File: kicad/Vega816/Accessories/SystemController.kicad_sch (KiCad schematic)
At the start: 3 parts, among them J102 VIA Port

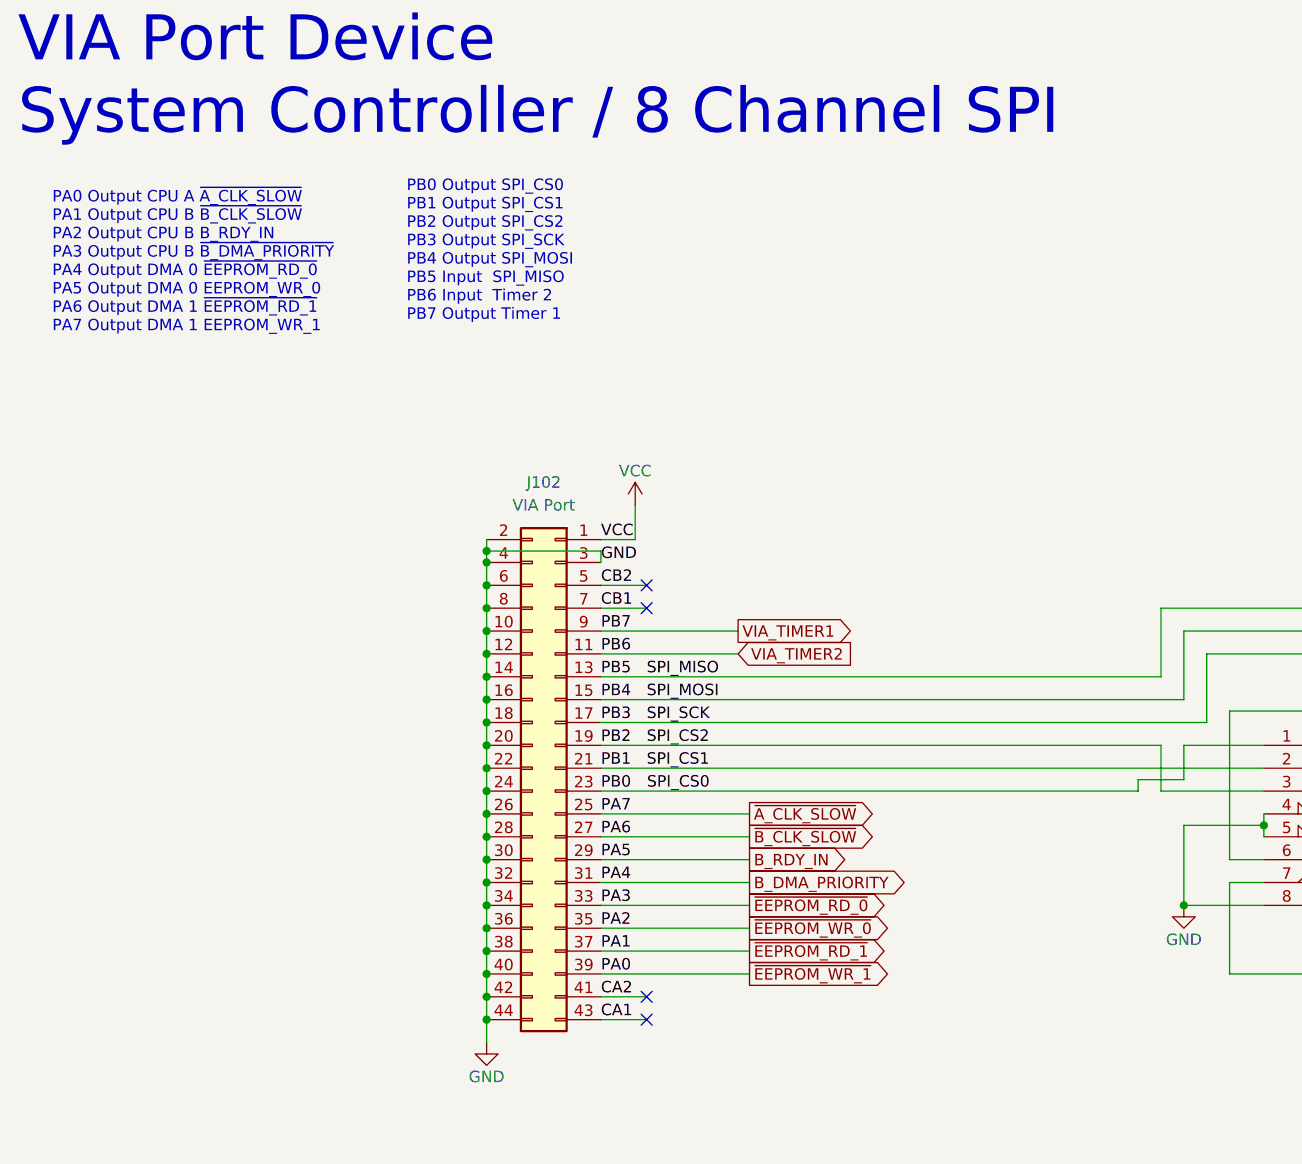
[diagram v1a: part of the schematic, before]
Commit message: expansion port hi ram
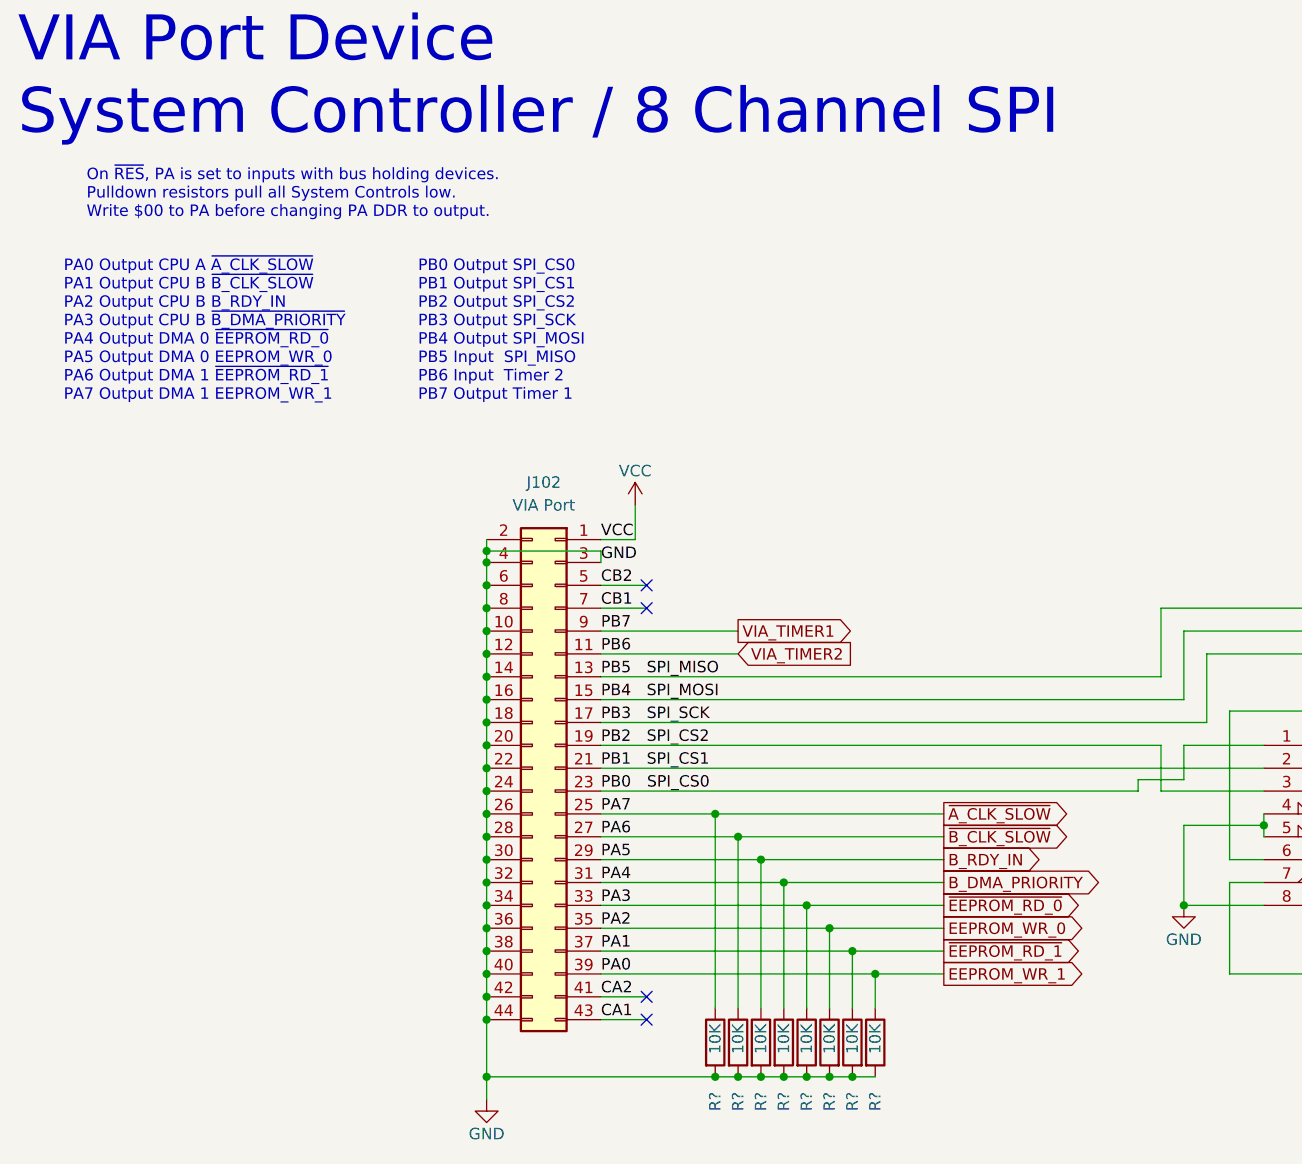
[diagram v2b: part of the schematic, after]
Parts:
- added R? (x8): 10K, symbol Device:R
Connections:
- net B_DMA_PRIORITY: now also R?.1
- net B_RDY_IN: now also R?.1
- net GND: now also R?.2, R?.2, R?.2, R?.2, R?.2, R?.2, R?.2, R?.2
- net ~{A_CLK_SLOW}: now also R?.1
- net ~{B_CLK_SLOW}: now also R?.1
- net ~{EEPROM_RD_0}: now also R?.1
- net ~{EEPROM_RD_1}: now also R?.1
- net ~{EEPROM_WR_0} renamed EEPROM_WR_0
- net EEPROM_WR_0: now also R?.1
- net ~{EEPROM_WR_1} renamed EEPROM_WR_1
- net EEPROM_WR_1: now also R?.1
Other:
- note added: "On ~{RES}, PA is set to inputs with bus holding devices. Pulldown resistors pull all System Controls low. Write $00 to PA before changing PA DDR to output."

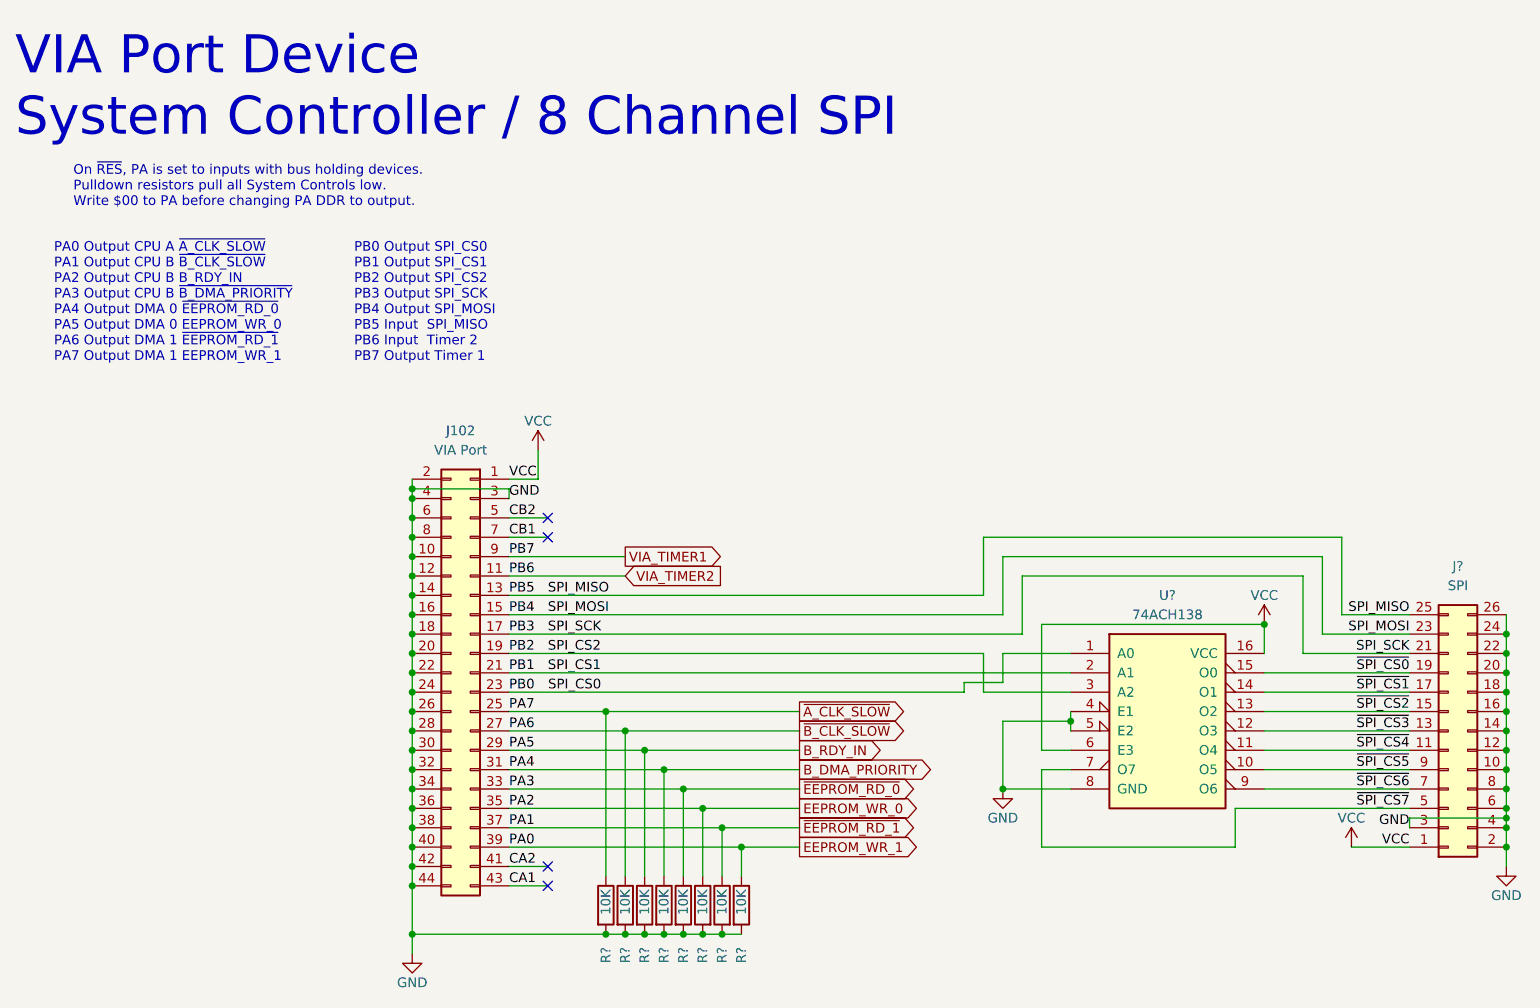
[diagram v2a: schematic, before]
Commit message: new plots
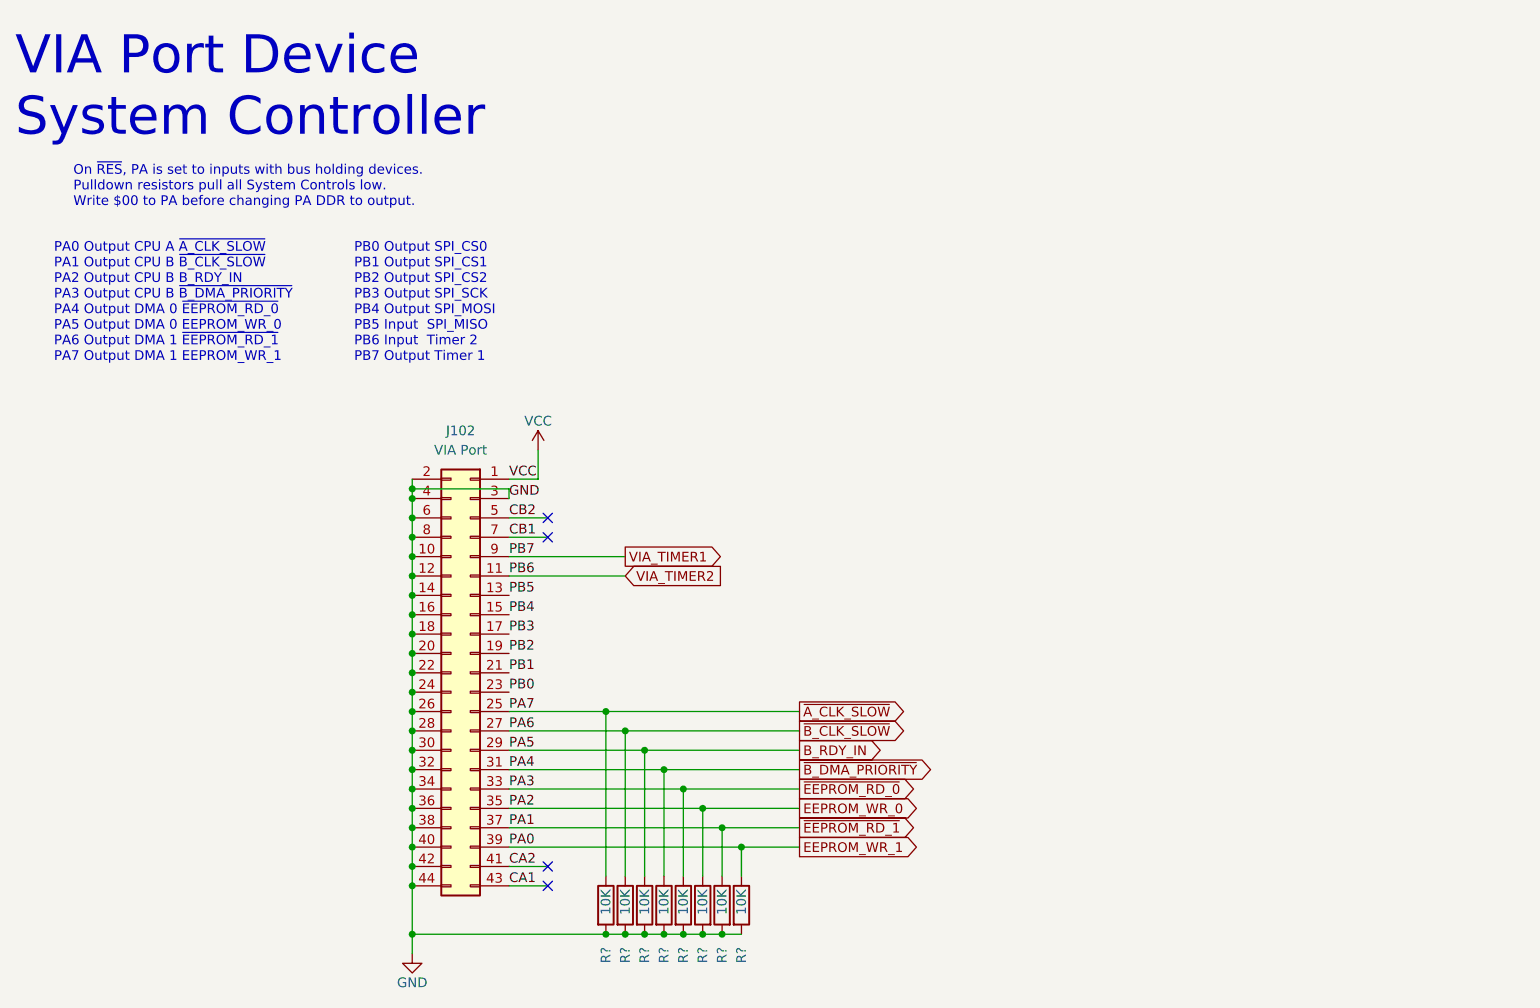
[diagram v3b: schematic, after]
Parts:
- removed J?: SPI, symbol Connector_Generic:Conn_02x13_Odd_Even
- removed U?: 74ACH138, symbol Vega816:74ACH138
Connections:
- net B_DMA_PRIORITY renamed ~{B_DMA_PRIORITY}
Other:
- note added: "VIA Port Device System Controller"
- note removed: "VIA Port Device System Controller / 8 Channel SPI"

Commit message: Big push, Sysctl, DMA Reg
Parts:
- removed R? (x8): 10K, symbol Device:R
- added J1: Sysctrl $7, Connector_PinHeader_2.54mm:PinHeader_2x08_P2.54mm_Vertical, symbol Vega816:Conn_02x08_Odd_Even
- added J10: Sysctrl $A, Connector_PinHeader_2.54mm:PinHeader_2x08_P2.54mm_Vertical, symbol Vega816:Conn_02x08_Odd_Even
- added J11: Sysctrl $B, Connector_PinHeader_2.54mm:PinHeader_2x08_P2.54mm_Vertical, symbol Vega816:Conn_02x08_Odd_Even
- added J12: Sysctrl $C, Connector_PinHeader_2.54mm:PinHeader_2x08_P2.54mm_Vertical, symbol Vega816:Conn_02x08_Odd_Even
- added J13: Sysctrl $D, Connector_PinHeader_2.54mm:PinHeader_2x08_P2.54mm_Vertical, symbol Vega816:Conn_02x08_Odd_Even
- added J16: Sysctrl $E, Connector_PinHeader_2.54mm:PinHeader_2x08_P2.54mm_Vertical, symbol Vega816:Conn_02x08_Odd_Even
- added J17: Sysctrl $F, Connector_PinHeader_2.54mm:PinHeader_2x08_P2.54mm_Vertical, symbol Vega816:Conn_02x08_Odd_Even
- added J18: Sysctrl $8, Connector_PinHeader_2.54mm:PinHeader_2x08_P2.54mm_Vertical, symbol Vega816:Conn_02x08_Odd_Even
- added J2: Sysctrl $6, Connector_PinHeader_2.54mm:PinHeader_2x08_P2.54mm_Vertical, symbol Vega816:Conn_02x08_Odd_Even
- added J3: Sysctrl $5, Connector_PinHeader_2.54mm:PinHeader_2x08_P2.54mm_Vertical, symbol Vega816:Conn_02x08_Odd_Even
- added J4: Sysctrl $4, Connector_PinHeader_2.54mm:PinHeader_2x08_P2.54mm_Vertical, symbol Vega816:Conn_02x08_Odd_Even
- added J5: Sysctrl $3, Connector_PinHeader_2.54mm:PinHeader_2x08_P2.54mm_Vertical, symbol Vega816:Conn_02x08_Odd_Even
- added J6: Sysctrl $2, Connector_PinHeader_2.54mm:PinHeader_2x08_P2.54mm_Vertical, symbol Vega816:Conn_02x08_Odd_Even
- added J7: Sysctrl $1, Connector_PinHeader_2.54mm:PinHeader_2x08_P2.54mm_Vertical, symbol Vega816:Conn_02x08_Odd_Even
- added J8: Sysctrl $0, Connector_PinHeader_2.54mm:PinHeader_2x08_P2.54mm_Vertical, symbol Vega816:Conn_02x08_Odd_Even
- added J9: Sysctrl $9, Connector_PinHeader_2.54mm:PinHeader_2x08_P2.54mm_Vertical, symbol Vega816:Conn_02x08_Odd_Even
- added U11, U18, U22, U32, U49, U53, U57, U6: 74HC32, Package_DIP:DIP-14_W7.62mm_Socket, symbol Vega816:74HC32
- added U15, U20, U30, U47, U5, U51, U55, U59: 74HC259, symbol Vega816:74HC259
- added U17, U48, U60, U63, U67, U70, U73, U?: 74HC373, symbol 74xx:74HC373
- added U2, U3: 74ACH138, Package_DIP:DIP-14_W7.62mm_Socket, symbol Vega816:74ACH138
- added U21, U52, U61, U65, U68, U7, U71, U74: 74HC02, symbol 74xx:74HC02
- added U4: 74HC04, symbol 74xx:74HC04
- added U? (x16): 74HC541, symbol Vega816:74HC541
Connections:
- net GND: now also J10.10 (Pin_10), J10.12 (Pin_12), J10.14 (Pin_14), J10.16 (Pin_16), J10.2 (Pin_2), J10.4 (Pin_4), J10.6 (Pin_6), J10.8 (Pin_8), J11.10 (Pin_10), J11.12 (Pin_12), J11.14 (Pin_14), J11.16 (Pin_16), J11.2 (Pin_2), J11.4 (Pin_4), J11.6 (Pin_6), J11.8 (Pin_8), J12.10 (Pin_10), J12.12 (Pin_12), J12.14 (Pin_14), J12.16 (Pin_16), J12.2 (Pin_2), J12.4 (Pin_4), J12.6 (Pin_6), J12.8 (Pin_8), J13.10 (Pin_10), J13.12 (Pin_12), J13.14 (Pin_14), J13.16 (Pin_16), J13.2 (Pin_2), J13.4 (Pin_4), J13.6 (Pin_6), J13.8 (Pin_8), J16.10 (Pin_10), J16.12 (Pin_12), J16.14 (Pin_14), J16.16 (Pin_16), J16.2 (Pin_2), J16.4 (Pin_4), J16.6 (Pin_6), J16.8 (Pin_8), J17.10 (Pin_10), J17.12 (Pin_12), J17.14 (Pin_14), J17.16 (Pin_16), J17.2 (Pin_2), J17.4 (Pin_4), J17.6 (Pin_6), J17.8 (Pin_8), J18.10 (Pin_10), J18.12 (Pin_12), J18.14 (Pin_14), J18.16 (Pin_16), J18.2 (Pin_2), J18.4 (Pin_4), J18.6 (Pin_6), J18.8 (Pin_8), J4.10 (Pin_10), J4.12 (Pin_12), J4.14 (Pin_14), J4.16 (Pin_16), J4.2 (Pin_2), J4.4 (Pin_4), J4.6 (Pin_6), J4.8 (Pin_8), J8.10 (Pin_10), J8.12 (Pin_12), J8.14 (Pin_14), J8.16 (Pin_16), J8.2 (Pin_2), J8.4 (Pin_4), J8.6 (Pin_6), J8.8 (Pin_8), J9.10 (Pin_10), J9.12 (Pin_12), J9.14 (Pin_14), J9.16 (Pin_16), J9.2 (Pin_2), J9.4 (Pin_4), J9.6 (Pin_6), J9.8 (Pin_8), U15.8 (GND), U17.1 (OE), U17.10 (GND), U20.8 (GND), U30.8 (GND), U47.8 (GND), U48.1 (OE), U48.10 (GND), U5.8 (GND), U51.8 (GND), U55.8 (GND), U59.8 (GND), U60.1 (OE), U60.10 (GND), U63.1 (OE), U63.10 (GND), U67.1 (OE), U67.10 (GND), U70.1 (OE), U70.10 (GND), U73.1 (OE), U73.10 (GND), U?.1 (OE), U?.10 (GND), U?.10 (GND), U?.10 (GND), U?.10 (GND), U?.10 (GND), U?.10 (GND), U?.10 (GND), U?.10 (GND), U?.10 (GND), U?.10 (GND), U?.10 (GND), U?.10 (GND), U?.10 (GND), U?.10 (GND), U?.10 (GND), U?.10 (GND), U?.10 (GND)
- net VCC: now also U15.16 (VCC), U17.20 (VCC), U20.16 (VCC), U30.16 (VCC), U47.16 (VCC), U48.20 (VCC), U5.16 (VCC), U51.16 (VCC), U55.16 (VCC), U59.16 (VCC), U60.20 (VCC), U63.20 (VCC), U67.20 (VCC), U70.20 (VCC), U73.20 (VCC), U?.20 (VCC), U?.20 (VCC), U?.20 (VCC), U?.20 (VCC), U?.20 (VCC), U?.20 (VCC), U?.20 (VCC), U?.20 (VCC), U?.20 (VCC), U?.20 (VCC), U?.20 (VCC), U?.20 (VCC), U?.20 (VCC), U?.20 (VCC), U?.20 (VCC), U?.20 (VCC), U?.20 (VCC)
- net B_RDY_IN renamed PA5
- net PA5: now also U17.14 (D5), U48.14 (D5), U60.14 (D5), U63.14 (D5), U67.14 (D5), U70.14 (D5), U73.14 (D5), U?.13 (Y5), U?.13 (Y5), U?.13 (Y5), U?.13 (Y5), U?.13 (Y5), U?.13 (Y5), U?.13 (Y5), U?.13 (Y5), U?.14 (D5), U?.16 (Y2), U?.16 (Y2), U?.16 (Y2), U?.16 (Y2), U?.16 (Y2), U?.16 (Y2), U?.16 (Y2), U?.16 (Y2)
- net CA2 renamed CA2_~{LE}
- net CA2_~{LE}: now also U11.1, U21.3, U52.3, U6.1, U61.3, U65.3, U68.3, U7.3, U71.3, U74.3
- net CB2 renamed CB2_CLR
- net CB2_CLR: now also U15.15 (Clr), U20.15 (Clr), U30.15 (Clr), U47.15 (Clr), U5.15 (Clr), U51.15 (Clr), U55.15 (Clr), U59.15 (Clr)
- net EEPROM_WR_0 renamed PA2
- net PA2: now also U17.7 (D2), U48.7 (D2), U60.7 (D2), U63.7 (D2), U67.7 (D2), U70.7 (D2), U73.7 (D2), U?.13 (Y5), U?.13 (Y5), U?.13 (Y5), U?.13 (Y5), U?.13 (Y5), U?.13 (Y5), U?.13 (Y5), U?.13 (Y5), U?.16 (Y2), U?.16 (Y2), U?.16 (Y2), U?.16 (Y2), U?.16 (Y2), U?.16 (Y2), U?.16 (Y2), U?.16 (Y2), U?.7 (D2)
- net EEPROM_WR_1 renamed PA0_D
- net PA0_D: now also U15.13 (D), U17.3 (D0), U20.13 (D), U30.13 (D), U47.13 (D), U48.3 (D0), U5.13 (D), U51.13 (D), U55.13 (D), U59.13 (D), U60.3 (D0), U63.3 (D0), U67.3 (D0), U70.3 (D0), U73.3 (D0), U?.11 (Y7), U?.11 (Y7), U?.11 (Y7), U?.11 (Y7), U?.11 (Y7), U?.11 (Y7), U?.11 (Y7), U?.11 (Y7), U?.18 (Y0), U?.18 (Y0), U?.18 (Y0), U?.18 (Y0), U?.18 (Y0), U?.18 (Y0), U?.18 (Y0), U?.18 (Y0), U?.3 (D0)
- net PB0 renamed PB0_A0
- net PB0_A0: now also U15.1 (A0), U20.1 (A0), U30.1 (A0), U47.1 (A0), U5.1 (A0), U51.1 (A0), U55.1 (A0), U59.1 (A0)
- net PB1 renamed PB1_A1
- net PB1_A1: now also U15.2 (A1), U20.2 (A1), U30.2 (A1), U47.2 (A1), U5.2 (A1), U51.2 (A1), U55.2 (A1), U59.2 (A1)
- net PB2 renamed PB2_A2
- net PB2_A2: now also U15.3 (A2), U20.3 (A2), U30.3 (A2), U47.3 (A2), U5.3 (A2), U51.3 (A2), U55.3 (A2), U59.3 (A2)
- net PB3 renamed PB3_A3
- net PB3_A3: now also U2.1 (A0), U3.1 (A0)
- net PB4 renamed PB4_A4
- net PB4_A4: now also U2.2 (A1), U3.2 (A1)
- net PB5 renamed PB5_A5
- net PB5_A5: now also U2.3 (A2), U3.3 (A2)
- net VIA_TIMER1 renamed PB7_RD
- net PB7_RD: now also U4.1
- net VIA_TIMER2 renamed PB6_A6
- net PB6_A6: now also U2.4 (E1), U3.6 (E3)
- net ~{A_CLK_SLOW} renamed PA7
- net PA7: now also U17.18 (D7), U48.18 (D7), U60.18 (D7), U63.18 (D7), U67.18 (D7), U70.18 (D7), U73.18 (D7), U?.11 (Y7), U?.11 (Y7), U?.11 (Y7), U?.11 (Y7), U?.11 (Y7), U?.11 (Y7), U?.11 (Y7), U?.11 (Y7), U?.18 (D7), U?.18 (Y0), U?.18 (Y0), U?.18 (Y0), U?.18 (Y0), U?.18 (Y0), U?.18 (Y0), U?.18 (Y0), U?.18 (Y0)
- net ~{B_CLK_SLOW} renamed PA6
- net PA6: now also U17.17 (D6), U48.17 (D6), U60.17 (D6), U63.17 (D6), U67.17 (D6), U70.17 (D6), U73.17 (D6), U?.12 (Y6), U?.12 (Y6), U?.12 (Y6), U?.12 (Y6), U?.12 (Y6), U?.12 (Y6), U?.12 (Y6), U?.12 (Y6), U?.17 (D6), U?.17 (Y1), U?.17 (Y1), U?.17 (Y1), U?.17 (Y1), U?.17 (Y1), U?.17 (Y1), U?.17 (Y1), U?.17 (Y1)
- net ~{B_DMA_PRIORITY} renamed PA4
- net PA4: now also U17.13 (D4), U48.13 (D4), U60.13 (D4), U63.13 (D4), U67.13 (D4), U70.13 (D4), U73.13 (D4), U?.13 (D4), U?.14 (Y4), U?.14 (Y4), U?.14 (Y4), U?.14 (Y4), U?.14 (Y4), U?.14 (Y4), U?.14 (Y4), U?.14 (Y4), U?.15 (Y3), U?.15 (Y3), U?.15 (Y3), U?.15 (Y3), U?.15 (Y3), U?.15 (Y3), U?.15 (Y3), U?.15 (Y3)
- net ~{EEPROM_RD_0} renamed PA3
- net PA3: now also U17.8 (D3), U48.8 (D3), U60.8 (D3), U63.8 (D3), U67.8 (D3), U70.8 (D3), U73.8 (D3), U?.14 (Y4), U?.14 (Y4), U?.14 (Y4), U?.14 (Y4), U?.14 (Y4), U?.14 (Y4), U?.14 (Y4), U?.14 (Y4), U?.15 (Y3), U?.15 (Y3), U?.15 (Y3), U?.15 (Y3), U?.15 (Y3), U?.15 (Y3), U?.15 (Y3), U?.15 (Y3), U?.8 (D3)
- net ~{EEPROM_RD_1} renamed PA1
- net PA1: now also U17.4 (D1), U48.4 (D1), U60.4 (D1), U63.4 (D1), U67.4 (D1), U70.4 (D1), U73.4 (D1), U?.12 (Y6), U?.12 (Y6), U?.12 (Y6), U?.12 (Y6), U?.12 (Y6), U?.12 (Y6), U?.12 (Y6), U?.12 (Y6), U?.17 (Y1), U?.17 (Y1), U?.17 (Y1), U?.17 (Y1), U?.17 (Y1), U?.17 (Y1), U?.17 (Y1), U?.17 (Y1), U?.4 (D1)
- new net: J5.1 (Pin_1), U47.12 (Q7)
- new net: J5.10 (Pin_10), U?.5 (A3)
- new net: J5.11 (Pin_11), U47.6 (Q2)
- new net: J5.12 (Pin_12), U?.4 (A2)
- new net: J5.13 (Pin_13), U47.5 (Q1)
- new net: J5.14 (Pin_14), U?.3 (A1)
- new net: J5.15 (Pin_15), U47.4 (Q0)
- new net: J5.16 (Pin_16), U?.2 (A0)
- new net: J5.2 (Pin_2), U?.9 (A7)
- new net: J5.3 (Pin_3), U47.11 (Q6)
- new net: J5.4 (Pin_4), U?.8 (A6)
- new net: J5.5 (Pin_5), U47.10 (Q5)
- new net: J5.6 (Pin_6), U?.7 (A5)
- new net: J5.7 (Pin_7), U47.9 (Q4)
- new net: J5.8 (Pin_8), U?.6 (A4)
- new net: J5.9 (Pin_9), U47.7 (Q3)
- new net: U2.14 (O1), U53.2, U?.1 (G1)
- new net: U4.2, U?.19 (G2), U?.19 (G2), U?.19 (G2), U?.19 (G2), U?.19 (G2), U?.19 (G2), U?.19 (G2), U?.19 (G2), U?.19 (G2), U?.19 (G2), U?.19 (G2), U?.19 (G2), U?.19 (G2), U?.19 (G2), U?.19 (G2), U?.19 (G2)
- new net: J7.16 (Pin_16), U?.2 (A0)
- new net: J7.14 (Pin_14), U?.3 (A1)
- new net: J7.12 (Pin_12), U?.4 (A2)
- new net: J7.10 (Pin_10), U?.5 (A3)
- new net: J7.8 (Pin_8), U?.6 (A4)
- new net: J7.6 (Pin_6), U?.7 (A5)
- new net: J7.4 (Pin_4), U?.8 (A6)
- new net: J7.2 (Pin_2), U?.9 (A7)
- new net: U3.15 (O0), U7.2, U?.1 (G1)
- new net: J18.1 (Pin_1), U?.2 (A0), U?.2 (O0)
- new net: J18.3 (Pin_3), U?.3 (A1), U?.5 (O1)
- new net: J18.5 (Pin_5), U?.4 (A2), U?.6 (O2)
- new net: J18.7 (Pin_7), U?.5 (A3), U?.9 (O3)
- new net: J18.9 (Pin_9), U?.12 (O4), U?.6 (A4)
- new net: J18.11 (Pin_11), U?.15 (O5), U?.7 (A5)
- new net: J18.13 (Pin_13), U?.16 (O6), U?.8 (A6)
- new net: J18.15 (Pin_15), U?.19 (O7), U?.9 (A7)
- new net: U60.11 (LE), U61.1
- new net: J11.9 (Pin_9), U60.12 (O4), U?.6 (A4)
- new net: J11.11 (Pin_11), U60.15 (O5), U?.7 (A5)
- new net: J11.13 (Pin_13), U60.16 (O6), U?.8 (A6)
- new net: J11.15 (Pin_15), U60.19 (O7), U?.9 (A7)
- new net: J11.1 (Pin_1), U60.2 (O0), U?.2 (A0)
- new net: J11.3 (Pin_3), U60.5 (O1), U?.3 (A1)
- new net: J11.5 (Pin_5), U60.6 (O2), U?.4 (A2)
- new net: J11.7 (Pin_7), U60.9 (O3), U?.5 (A3)
- new net: U11.2, U2.9 (O6), U?.1 (G1)
- new net: U11.3, U15.14 (E)
- new net: U17.11 (LE), U21.1
- new net: J9.9 (Pin_9), U17.12 (O4), U?.6 (A4)
- new net: J9.11 (Pin_11), U17.15 (O5), U?.7 (A5)
- new net: J9.13 (Pin_13), U17.16 (O6), U?.8 (A6)
- new net: J9.15 (Pin_15), U17.19 (O7), U?.9 (A7)
- new net: J9.1 (Pin_1), U17.2 (O0), U?.2 (A0)
- new net: J9.3 (Pin_3), U17.5 (O1), U?.3 (A1)
- new net: J9.5 (Pin_5), U17.6 (O2), U?.4 (A2)
- new net: J9.7 (Pin_7), U17.9 (O3), U?.5 (A3)
- new net: U18.2, U2.10 (O5), U?.1 (G1)
- new net: U2.11 (O4), U22.2, U?.1 (G1)
- new net: U2.12 (O3), U32.2, U?.1 (G1)
- new net: U2.13 (O2), U49.2, U?.1 (G1)
- new net: U2.15 (O0), U57.2, U?.1 (G1)
- new net: U2.16 (VCC), U2.6 (E3)
- new net: U2.5 (E2), U2.8 (GND)
- new net: U2.7 (O7), U6.2, U?.1 (G1)
- new net: J7.1 (Pin_1), U55.12 (Q7)
- new net: J7.11 (Pin_11), U55.6 (Q2)
- new net: J7.13 (Pin_13), U55.5 (Q1)
- new net: J7.15 (Pin_15), U55.4 (Q0)
- new net: J7.3 (Pin_3), U55.11 (Q6)
- new net: J7.5 (Pin_5), U55.10 (Q5)
- new net: J7.7 (Pin_7), U55.9 (Q4)
- new net: J7.9 (Pin_9), U55.7 (Q3)
- new net: U18.1, U22.1, U32.1, U49.1
- new net: U22.3, U30.14 (E)
- new net: U3.10 (O5), U68.2, U?.1 (G1)
- new net: J13.1 (Pin_1), U67.2 (O0), U?.2 (A0)
- new net: J13.3 (Pin_3), U67.5 (O1), U?.3 (A1)
- new net: J13.5 (Pin_5), U67.6 (O2), U?.4 (A2)
- new net: J13.7 (Pin_7), U67.9 (O3), U?.5 (A3)
- new net: J13.9 (Pin_9), U67.12 (O4), U?.6 (A4)
- new net: J13.11 (Pin_11), U67.15 (O5), U?.7 (A5)
- new net: J13.13 (Pin_13), U67.16 (O6), U?.8 (A6)
- new net: J13.15 (Pin_15), U67.19 (O7), U?.9 (A7)
- new net: J2.16 (Pin_16), U?.2 (A0)
- new net: J2.14 (Pin_14), U?.3 (A1)
- new net: J2.12 (Pin_12), U?.4 (A2)
- new net: J2.10 (Pin_10), U?.5 (A3)
- new net: J2.8 (Pin_8), U?.6 (A4)
- new net: J2.6 (Pin_6), U?.7 (A5)
- new net: J2.4 (Pin_4), U?.8 (A6)
- new net: J2.2 (Pin_2), U?.9 (A7)
- new net: U21.2, U3.14 (O1), U?.1 (G1)
- new net: J2.5 (Pin_5), U15.10 (Q5)
- new net: J2.3 (Pin_3), U15.11 (Q6)
- new net: J2.1 (Pin_1), U15.12 (Q7)
- new net: J2.15 (Pin_15), U15.4 (Q0)
- new net: J2.13 (Pin_13), U15.5 (Q1)
- new net: J2.11 (Pin_11), U15.6 (Q2)
- new net: J2.9 (Pin_9), U15.7 (Q3)
- new net: J2.7 (Pin_7), U15.9 (Q4)
- new net: U3.12 (O3), U61.2, U?.1 (G1)
- new net: U53.1, U57.1
- new net: U53.3, U55.14 (E)
- new net: J8.15 (Pin_15), U59.4 (Q0), U?.2 (A0)
- new net: J8.13 (Pin_13), U59.5 (Q1), U?.3 (A1)
- new net: J8.11 (Pin_11), U59.6 (Q2), U?.4 (A2)
- new net: J8.9 (Pin_9), U59.7 (Q3), U?.5 (A3)
- new net: J8.7 (Pin_7), U59.9 (Q4), U?.6 (A4)
- new net: J8.5 (Pin_5), U59.10 (Q5), U?.7 (A5)
- new net: J8.3 (Pin_3), U59.11 (Q6), U?.8 (A6)
- new net: J8.1 (Pin_1), U59.12 (Q7), U?.9 (A7)
- new net: U67.11 (LE), U68.1
- new net: U18.3, U20.14 (E)
- new net: U32.3, U47.14 (E)
- new net: U3.9 (O6), U71.2, U?.1 (G1)
- new net: J16.1 (Pin_1), U70.2 (O0), U?.2 (A0)
- new net: J16.3 (Pin_3), U70.5 (O1), U?.3 (A1)
- new net: J16.5 (Pin_5), U70.6 (O2), U?.4 (A2)
- new net: J16.7 (Pin_7), U70.9 (O3), U?.5 (A3)
- new net: J16.9 (Pin_9), U70.12 (O4), U?.6 (A4)
- new net: J16.11 (Pin_11), U70.15 (O5), U?.7 (A5)
- new net: J16.13 (Pin_13), U70.16 (O6), U?.8 (A6)
- new net: J16.15 (Pin_15), U70.19 (O7), U?.9 (A7)
- new net: J12.1 (Pin_1), U63.2 (O0), U?.2 (A0)
- new net: J12.11 (Pin_11), U63.15 (O5), U?.7 (A5)
- new net: J12.13 (Pin_13), U63.16 (O6), U?.8 (A6)
- new net: J12.15 (Pin_15), U63.19 (O7), U?.9 (A7)
- new net: J12.3 (Pin_3), U63.5 (O1), U?.3 (A1)
- new net: J12.5 (Pin_5), U63.6 (O2), U?.4 (A2)
- new net: J12.7 (Pin_7), U63.9 (O3), U?.5 (A3)
- new net: J12.9 (Pin_9), U63.12 (O4), U?.6 (A4)
- new net: J6.1 (Pin_1), U51.12 (Q7)
- new net: J6.10 (Pin_10), U?.5 (A3)
- new net: J6.11 (Pin_11), U51.6 (Q2)
- new net: J6.12 (Pin_12), U?.4 (A2)
- new net: J6.13 (Pin_13), U51.5 (Q1)
- new net: J6.14 (Pin_14), U?.3 (A1)
- new net: J6.15 (Pin_15), U51.4 (Q0)
- new net: J6.16 (Pin_16), U?.2 (A0)
- new net: J6.2 (Pin_2), U?.9 (A7)
- new net: J6.3 (Pin_3), U51.11 (Q6)
- new net: J6.4 (Pin_4), U?.8 (A6)
- new net: J6.5 (Pin_5), U51.10 (Q5)
- new net: J6.6 (Pin_6), U?.7 (A5)
- new net: J6.7 (Pin_7), U51.9 (Q4)
- new net: J6.8 (Pin_8), U?.6 (A4)
- new net: J6.9 (Pin_9), U51.7 (Q3)
- new net: J10.1 (Pin_1), U48.2 (O0), U?.2 (A0)
- new net: J10.11 (Pin_11), U48.15 (O5), U?.7 (A5)
- new net: J10.13 (Pin_13), U48.16 (O6), U?.8 (A6)
- new net: J10.15 (Pin_15), U48.19 (O7), U?.9 (A7)
- new net: J10.3 (Pin_3), U48.5 (O1), U?.3 (A1)
- new net: J10.5 (Pin_5), U48.6 (O2), U?.4 (A2)
- new net: J10.7 (Pin_7), U48.9 (O3), U?.5 (A3)
- new net: J10.9 (Pin_9), U48.12 (O4), U?.6 (A4)
- new net: J3.1 (Pin_1), U20.12 (Q7)
- new net: J3.10 (Pin_10), U?.5 (A3)
- new net: J3.11 (Pin_11), U20.6 (Q2)
- new net: J3.12 (Pin_12), U?.4 (A2)
- new net: J3.13 (Pin_13), U20.5 (Q1)
- new net: J3.14 (Pin_14), U?.3 (A1)
- new net: J3.15 (Pin_15), U20.4 (Q0)
- new net: J3.16 (Pin_16), U?.2 (A0)
- new net: J3.2 (Pin_2), U?.9 (A7)
- new net: J3.3 (Pin_3), U20.11 (Q6)
- new net: J3.4 (Pin_4), U?.8 (A6)
- new net: J3.5 (Pin_5), U20.10 (Q5)
- new net: J3.6 (Pin_6), U?.7 (A5)
- new net: J3.7 (Pin_7), U20.9 (Q4)
- new net: J3.8 (Pin_8), U?.6 (A4)
- new net: J3.9 (Pin_9), U20.7 (Q3)
- new net: U48.11 (LE), U52.1
- new net: U57.3, U59.14 (E)
- new net: J1.16 (Pin_16), U?.2 (A0)
- new net: J1.14 (Pin_14), U?.3 (A1)
- new net: J1.12 (Pin_12), U?.4 (A2)
- new net: J1.10 (Pin_10), U?.5 (A3)
- new net: J1.8 (Pin_8), U?.6 (A4)
- new net: J1.6 (Pin_6), U?.7 (A5)
- new net: J1.4 (Pin_4), U?.8 (A6)
- new net: J1.2 (Pin_2), U?.9 (A7)
- new net: U7.1, U?.11 (LE)
- new net: J4.1 (Pin_1), U30.12 (Q7), U?.9 (A7)
- new net: J4.11 (Pin_11), U30.6 (Q2), U?.4 (A2)
- new net: J4.13 (Pin_13), U30.5 (Q1), U?.3 (A1)
- new net: J4.15 (Pin_15), U30.4 (Q0), U?.2 (A0)
- new net: J4.3 (Pin_3), U30.11 (Q6), U?.8 (A6)
- new net: J4.5 (Pin_5), U30.10 (Q5), U?.7 (A5)
- new net: J4.7 (Pin_7), U30.9 (Q4), U?.6 (A4)
- new net: J4.9 (Pin_9), U30.7 (Q3), U?.5 (A3)
- new net: U3.11 (O4), U65.2, U?.1 (G1)
- new net: U3.7 (O7), U74.2, U?.1 (G1)
- new net: J17.1 (Pin_1), U73.2 (O0), U?.2 (A0)
- new net: J17.3 (Pin_3), U73.5 (O1), U?.3 (A1)
- new net: J17.5 (Pin_5), U73.6 (O2), U?.4 (A2)
- new net: J17.7 (Pin_7), U73.9 (O3), U?.5 (A3)
- new net: J17.9 (Pin_9), U73.12 (O4), U?.6 (A4)
- new net: J17.11 (Pin_11), U73.15 (O5), U?.7 (A5)
- new net: J17.13 (Pin_13), U73.16 (O6), U?.8 (A6)
- new net: J17.15 (Pin_15), U73.19 (O7), U?.9 (A7)
- new net: U3.13 (O2), U52.2, U?.1 (G1)
- new net: U3.4 (E1), U3.5 (E2), U3.8 (GND)
- new net: U63.11 (LE), U65.1
- new net: J1.1 (Pin_1), U5.12 (Q7)
- new net: J1.11 (Pin_11), U5.6 (Q2)
- new net: J1.13 (Pin_13), U5.5 (Q1)
- new net: J1.15 (Pin_15), U5.4 (Q0)
- new net: J1.3 (Pin_3), U5.11 (Q6)
- new net: J1.5 (Pin_5), U5.10 (Q5)
- new net: J1.7 (Pin_7), U5.9 (Q4)
- new net: J1.9 (Pin_9), U5.7 (Q3)
- new net: U70.11 (LE), U71.1
- new net: U49.3, U51.14 (E)
- new net: U73.11 (LE), U74.1
- new net: U5.14 (E), U6.3
- no-connect marks 4 -> 2
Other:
- note added: "Sysctrl Registers 16 x 8 bit latches (8 addressable) VIA Port Device"
- note removed: "On ~{RES}, PA is set to inputs with bus holding devices. Pulldown resistors pull all System Controls low. Write $00 to PA before changing PA DDR to output."
- note removed: "PA0 Output CPU A ~{A_CLK_SLOW} PA1 Output CPU B ~{B_CLK_SLOW} PA2 Output CPU B B_RDY_IN PA3 Output CPU B ~{B_DMA_PRIORITY} PA4 Output DMA 0 ~{EEPROM_RD_0} PA5 Output DMA 0 EEPROM_WR_0 PA6 Output DMA 1 ~{EEPROM_RD_1} PA7 Output DMA 1 EEPROM_WR_1"
- note removed: "PB0 Output SPI_CS0 PB1 Output SPI_CS1 PB2 Output SPI_CS2 PB3 Output SPI_SCK PB4 Output SPI_MOSI PB5 Input SPI_MISO PB6 Input Timer 2 PB7 Output Timer 1"
- note removed: "VIA Port Device System Controller"
- moved on the sheet: J102

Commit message: dfsg
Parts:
- removed J1: Sysctrl $7, Connector_PinHeader_2.54mm:PinHeader_2x08_P2.54mm_Vertical, symbol Vega816:Conn_02x08_Odd_Even
- removed J10: Sysctrl $A, Connector_PinHeader_2.54mm:PinHeader_2x08_P2.54mm_Vertical, symbol Vega816:Conn_02x08_Odd_Even
- removed J102: VIA Port, symbol Connector_Generic:Conn_02x22_Odd_Even
- removed J11: Sysctrl $B, Connector_PinHeader_2.54mm:PinHeader_2x08_P2.54mm_Vertical, symbol Vega816:Conn_02x08_Odd_Even
- removed J12: Sysctrl $C, Connector_PinHeader_2.54mm:PinHeader_2x08_P2.54mm_Vertical, symbol Vega816:Conn_02x08_Odd_Even
- removed J13: Sysctrl $D, Connector_PinHeader_2.54mm:PinHeader_2x08_P2.54mm_Vertical, symbol Vega816:Conn_02x08_Odd_Even
- removed J16: Sysctrl $E, Connector_PinHeader_2.54mm:PinHeader_2x08_P2.54mm_Vertical, symbol Vega816:Conn_02x08_Odd_Even
- removed J17: Sysctrl $F, Connector_PinHeader_2.54mm:PinHeader_2x08_P2.54mm_Vertical, symbol Vega816:Conn_02x08_Odd_Even
- removed J18: Sysctrl $8, Connector_PinHeader_2.54mm:PinHeader_2x08_P2.54mm_Vertical, symbol Vega816:Conn_02x08_Odd_Even
- removed J2: Sysctrl $6, Connector_PinHeader_2.54mm:PinHeader_2x08_P2.54mm_Vertical, symbol Vega816:Conn_02x08_Odd_Even
- removed J3: Sysctrl $5, Connector_PinHeader_2.54mm:PinHeader_2x08_P2.54mm_Vertical, symbol Vega816:Conn_02x08_Odd_Even
- removed J4: Sysctrl $4, Connector_PinHeader_2.54mm:PinHeader_2x08_P2.54mm_Vertical, symbol Vega816:Conn_02x08_Odd_Even
- removed J5: Sysctrl $3, Connector_PinHeader_2.54mm:PinHeader_2x08_P2.54mm_Vertical, symbol Vega816:Conn_02x08_Odd_Even
- removed J6: Sysctrl $2, Connector_PinHeader_2.54mm:PinHeader_2x08_P2.54mm_Vertical, symbol Vega816:Conn_02x08_Odd_Even
- removed J7: Sysctrl $1, Connector_PinHeader_2.54mm:PinHeader_2x08_P2.54mm_Vertical, symbol Vega816:Conn_02x08_Odd_Even
- removed J8: Sysctrl $0, Connector_PinHeader_2.54mm:PinHeader_2x08_P2.54mm_Vertical, symbol Vega816:Conn_02x08_Odd_Even
- removed J9: Sysctrl $9, Connector_PinHeader_2.54mm:PinHeader_2x08_P2.54mm_Vertical, symbol Vega816:Conn_02x08_Odd_Even
- removed U11, U18, U22, U32, U49, U53, U57, U6: 74HC32, Package_DIP:DIP-14_W7.62mm_Socket, symbol Vega816:74HC32
- removed U15, U20, U30, U47, U5, U51, U55, U59: 74HC259, symbol Vega816:74HC259
- removed U17, U48, U60, U63, U67, U70, U73, U?: 74HC373, symbol 74xx:74HC373
- removed U2, U3: 74ACH138, Package_DIP:DIP-14_W7.62mm_Socket, symbol Vega816:74ACH138
- removed U21, U52, U61, U65, U68, U7, U71, U74: 74HC02, symbol 74xx:74HC02
- removed U4: 74HC04, symbol 74xx:74HC04
- removed U? (x16): 74HC541, symbol Vega816:74HC541
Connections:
- no-connect marks 2 -> 0
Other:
- note removed: "Sysctrl Registers 16 x 8 bit latches (8 addressable) VIA Port Device"
